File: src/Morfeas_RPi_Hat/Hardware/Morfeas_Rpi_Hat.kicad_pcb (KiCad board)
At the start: 2 copper layers, 65 x 56 mm, 58 parts, among them J1 Con, J2 RPi_header, J5 RS_232, Q1 SUM110P06, Q2 SUM110P06, U1 DS3231, U2 TSR2-2450, U3 TLV70433, U4 SP3232, U5 24AA08, U6 MAX9611, U7 MAX9611

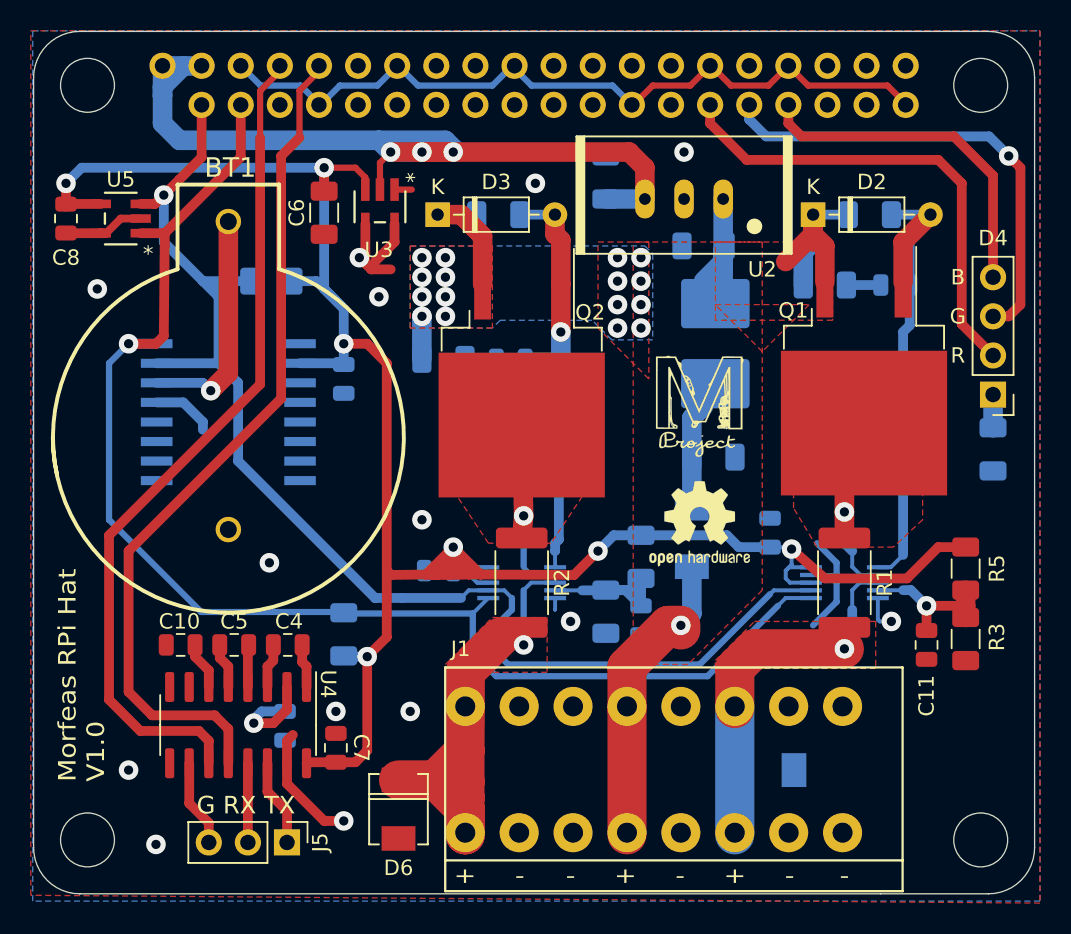
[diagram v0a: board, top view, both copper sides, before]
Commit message: Update Morfeas_RPi_Hat files
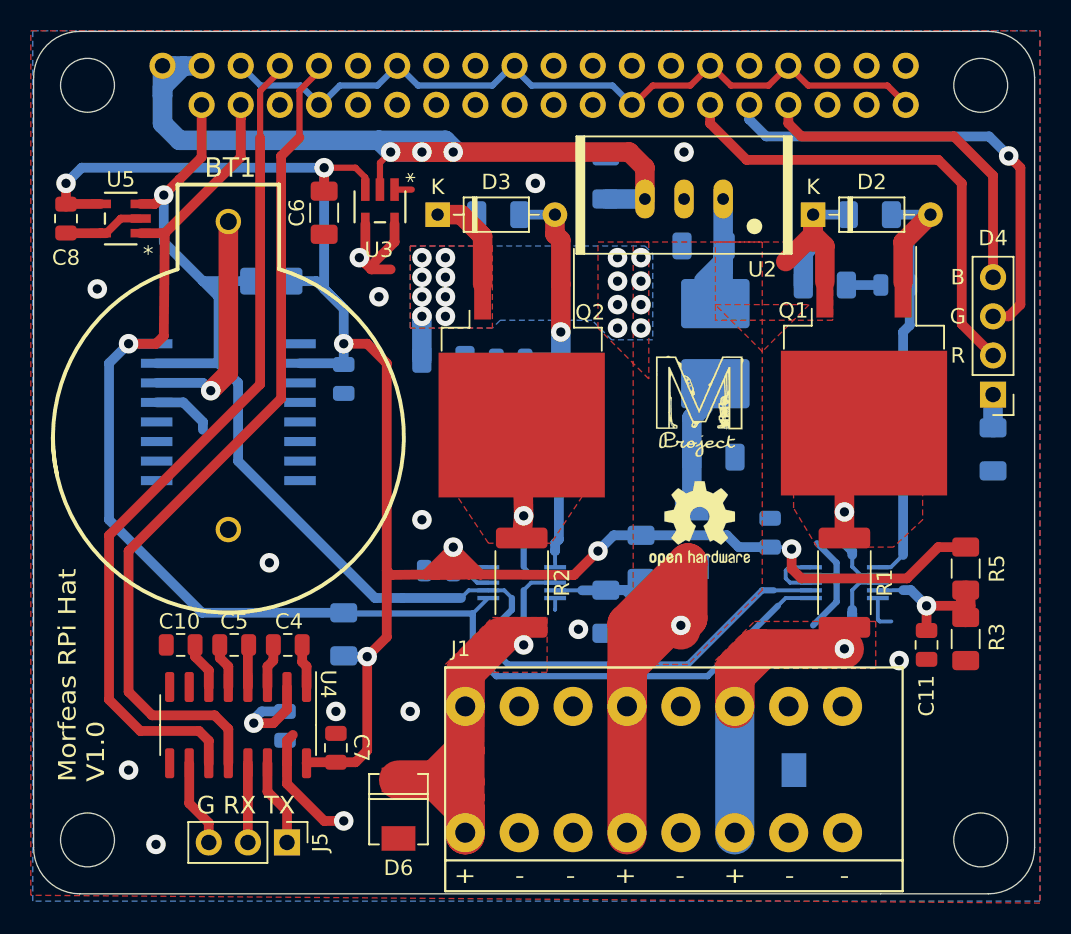
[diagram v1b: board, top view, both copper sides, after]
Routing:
- net SCL: track 89.7 -> 108.3 mm
- net +24V: track 51.7 -> 66.9 mm
- net /CAN0_P+: track 27.8 -> 33.0 mm
- net +3V3: track 143.3 -> 144.1 mm

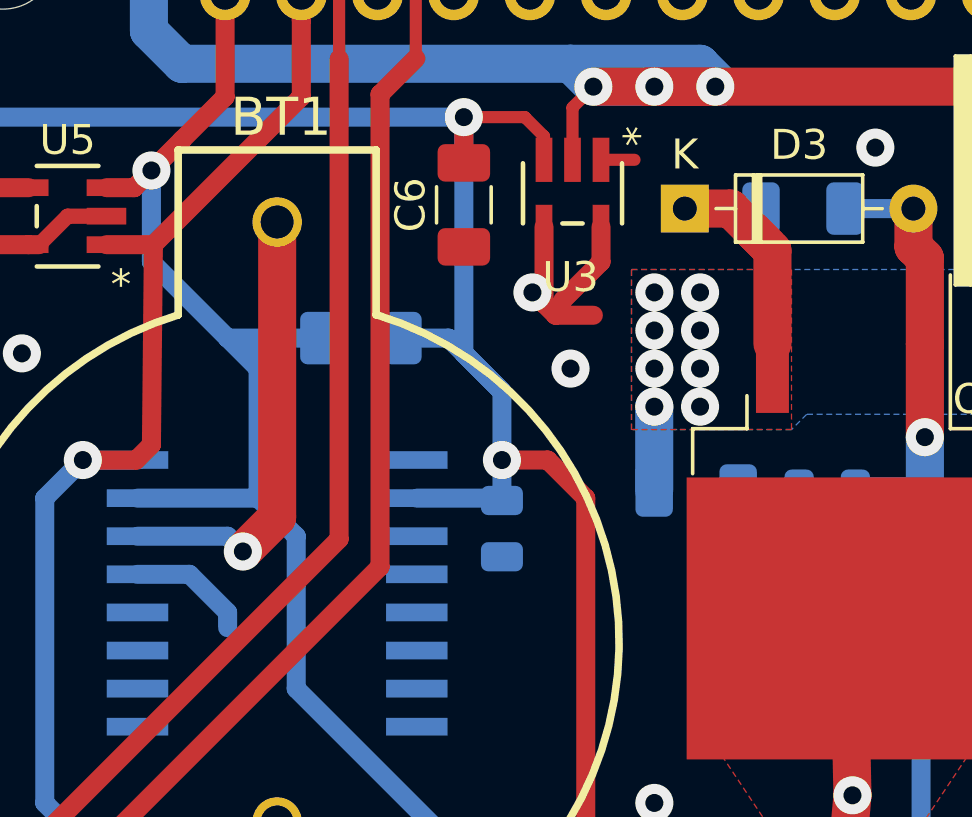
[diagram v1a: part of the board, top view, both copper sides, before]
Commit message: Update Morfeas_RPi_Hat files
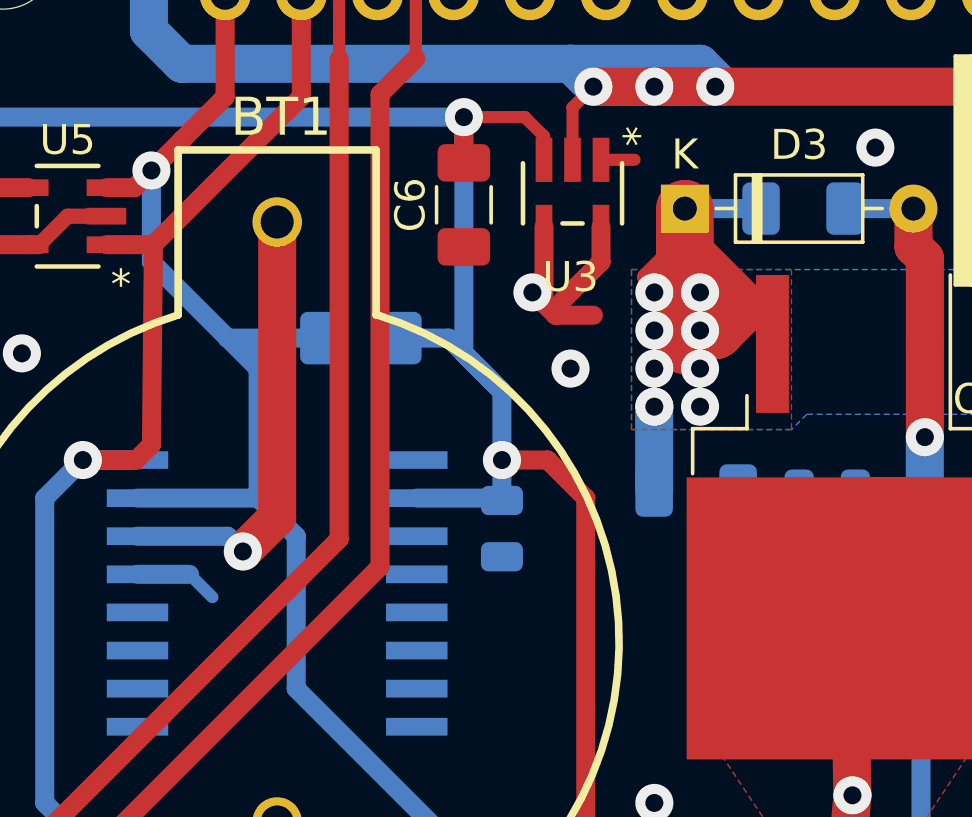
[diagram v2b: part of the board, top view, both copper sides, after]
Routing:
- net +24V: track 66.9 -> 69.9 mm
- net GND: track 93.8 -> 92.6 mm

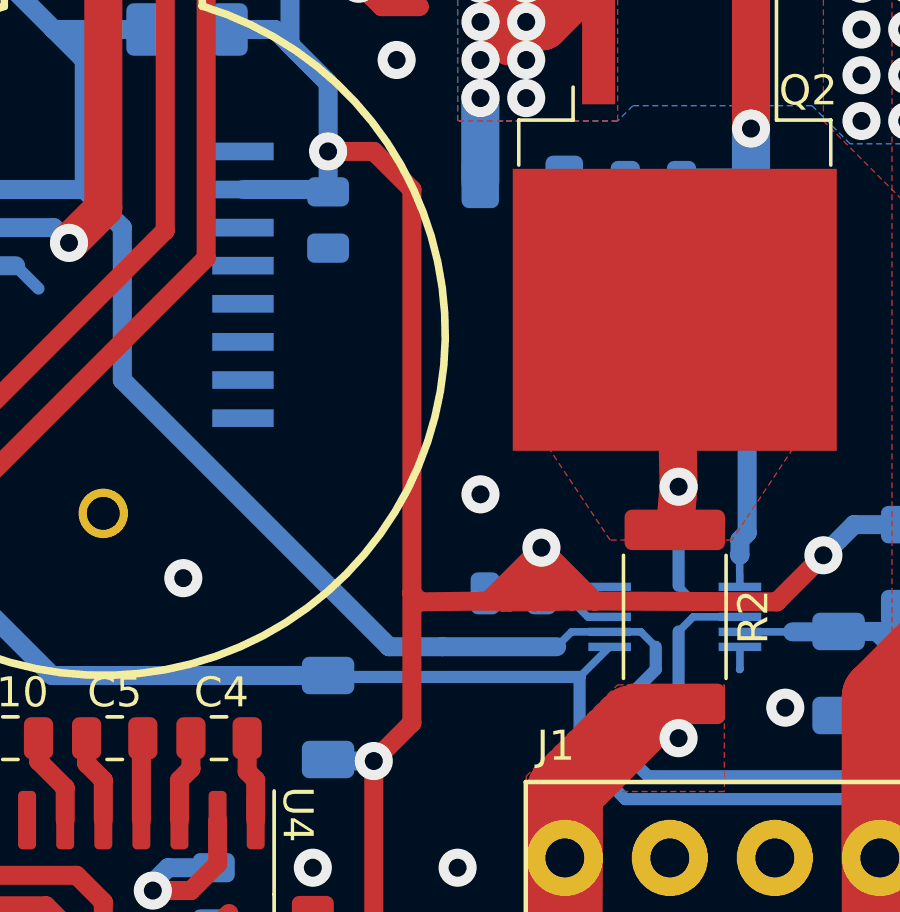
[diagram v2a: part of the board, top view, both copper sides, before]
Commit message: Update Morfeas_RPi_Hat files
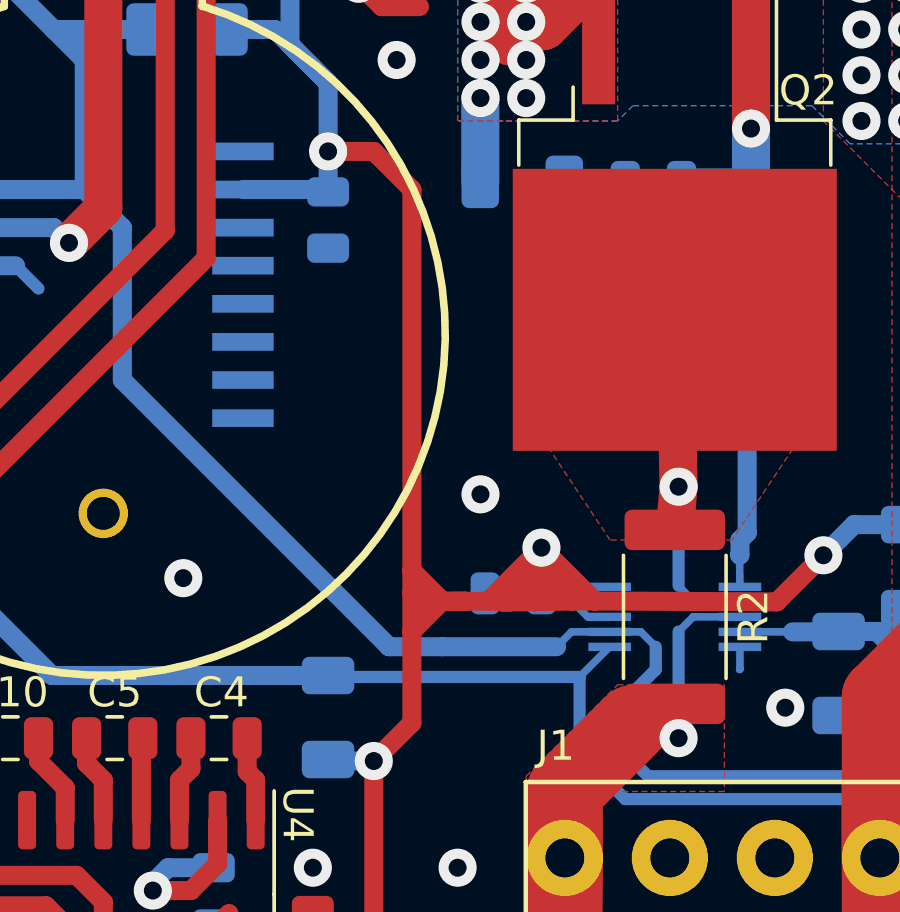
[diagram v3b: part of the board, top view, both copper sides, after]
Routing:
- net +3V3: track 144.1 -> 148.5 mm
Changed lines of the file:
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@@
     (thickness 1.6)
     (drawings 27)
-    (tracks 475)
+    (tracks 482)
     (zones 0)
     (modules 58)
@@
   (segment (start 143.256 104.14) (end 144.526 102.87) (width 0.635) (layer F.Cu) (net 10))
   (segment (start 144.809001 98.835001) (end 144.526 98.552) (width 0.635) (layer F.Cu) (net 10))
-  (segment (start 144.526 102.87) (end 144.526 98.552) (width 0.635) (layer F.Cu) (net 10))
   (segment (start 159.264 96.26) (end 158.242 97.282) (width 0.635) (layer B.Cu) (net 10))
   (segment (start 166.618 96.26) (end 159.264 96.26) (width 0.635) (layer B.Cu) (net 10))
@@
   (segment (start 148.844 97.028) (end 147.066 98.806) (width 0.635) (layer F.Cu) (net 10))
   (segment (start 147.544999 98.835001) (end 147.066 98.806) (width 0.635) (layer F.Cu) (net 10))
-  (segment (start 147.066 98.806) (end 144.809001 98.835001) (width 0.635) (layer F.Cu) (net 10))
   (segment (start 156.688999 98.835001) (end 150.622 98.806) (width 0.635) (layer F.Cu) (net 10))
   (segment (start 148.844 97.028) (end 150.622 98.806) (width 0.635) (layer F.Cu) (net 10))
@@
   (via (at 141.732 83.82) (size 1.27) (drill 0.6) (layers F.Cu B.Cu) (net 10))
   (segment (start 143.256 83.82) (end 141.732 83.82) (width 0.635) (layer F.Cu) (net 10))
-  (segment (start 144.526 98.552) (end 144.526 85.09) (width 0.635) (layer F.Cu) (net 10))
   (segment (start 144.526 85.09) (end 143.256 83.82) (width 0.635) (layer F.Cu) (net 10))
   (segment (start 139.381 110.998) (end 139.319 111.06) (width 0.635) (layer F.Cu) (net 10))
@@
   (segment (start 181.61 97.028) (end 180.34 97.028) (width 0.635) (layer F.Cu) (net 10))
   (segment (start 180.34 97.028) (end 178.308 99.06) (width 0.635) (layer F.Cu) (net 10))
+  (segment (start 146.313667 98.815667) (end 145.551667 98.815667) (width 0.635) (layer F.Cu) (net 10))
+  (segment (start 145.551667 98.815667) (end 144.526 97.79) (width 0.635) (layer F.Cu) (net 10))
+  (segment (start 146.313667 98.815667) (end 144.809001 98.835001) (width 0.635) (layer F.Cu) (net 10))
+  (segment (start 147.066 98.806) (end 146.313667 98.815667) (width 0.635) (layer F.Cu) (net 10))
+  (segment (start 144.526 97.79) (end 144.526 85.09) (width 0.635) (layer F.Cu) (net 10))
+  (segment (start 144.526 98.552) (end 144.526 97.79) (width 0.635) (layer F.Cu) (net 10))
+  (segment (start 145.532333 98.815667) (end 144.526 99.822) (width 0.635) (layer F.Cu) (net 10))
+  (segment (start 146.313667 98.815667) (end 145.532333 98.815667) (width 0.635) (layer F.Cu) (net 10))
+  (segment (start 144.526 102.87) (end 144.526 99.822) (width 0.635) (layer F.Cu) (net 10))
+  (segment (start 144.526 99.822) (end 144.526 98.552) (width 0.635) (layer F.Cu) (net 10))
   (via (at 135.89 108.458) (size 1.27) (drill 0.6) (layers F.Cu B.Cu) (net 11))
   (segment (start 136.398 107.696) (end 135.89 108.204) (width 0.635) (layer B.Cu) (net 11))
